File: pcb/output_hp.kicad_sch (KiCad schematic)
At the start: 1 part, among them J13 AudioJack3

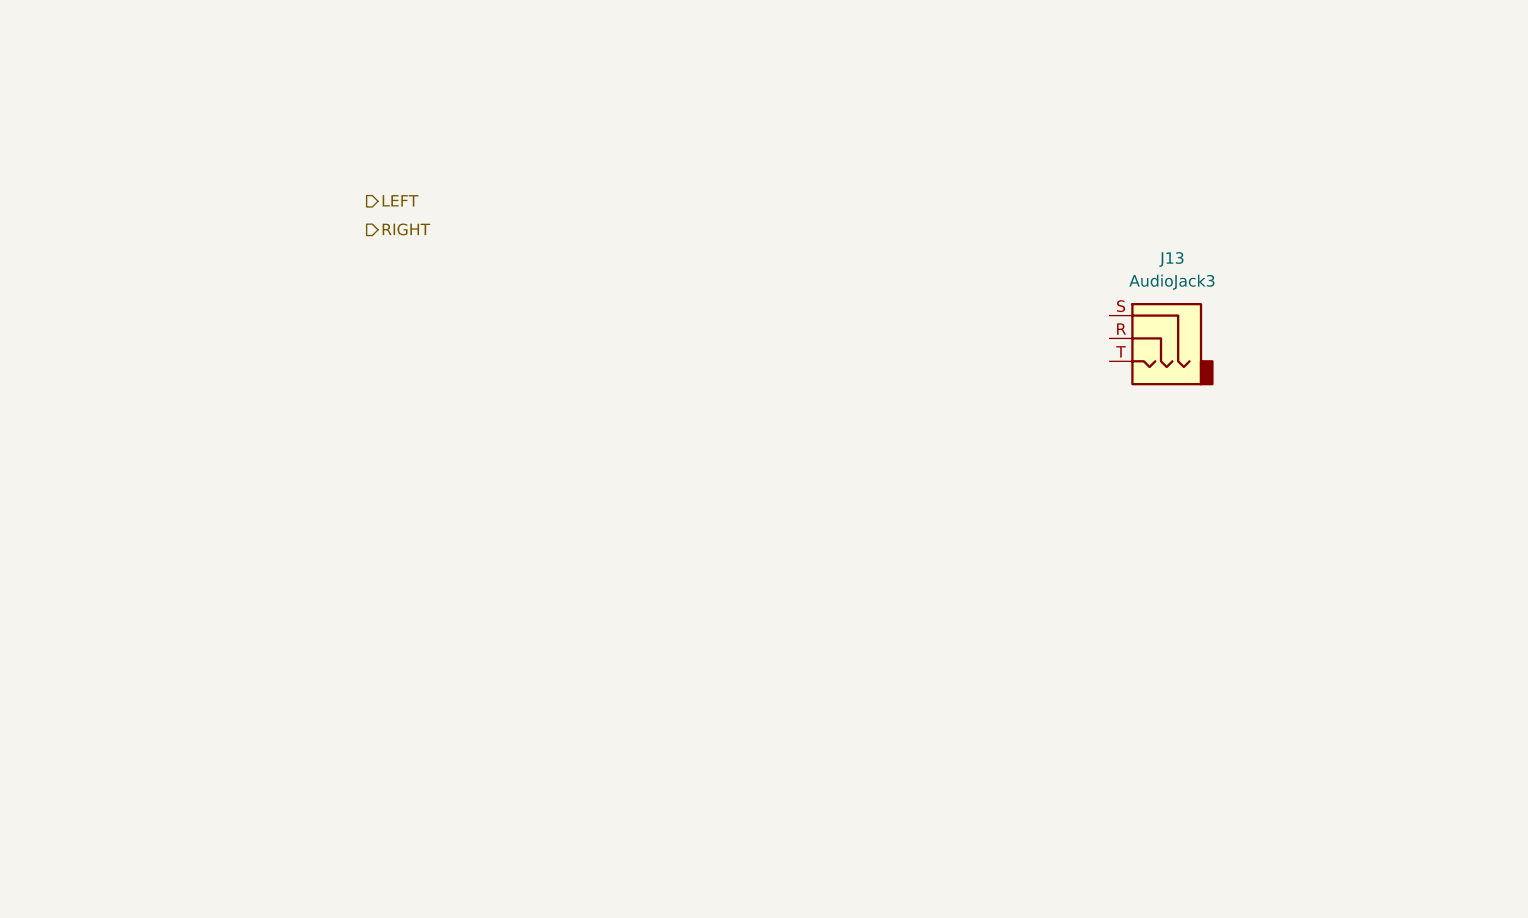
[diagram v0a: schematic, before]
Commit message: progress on hp
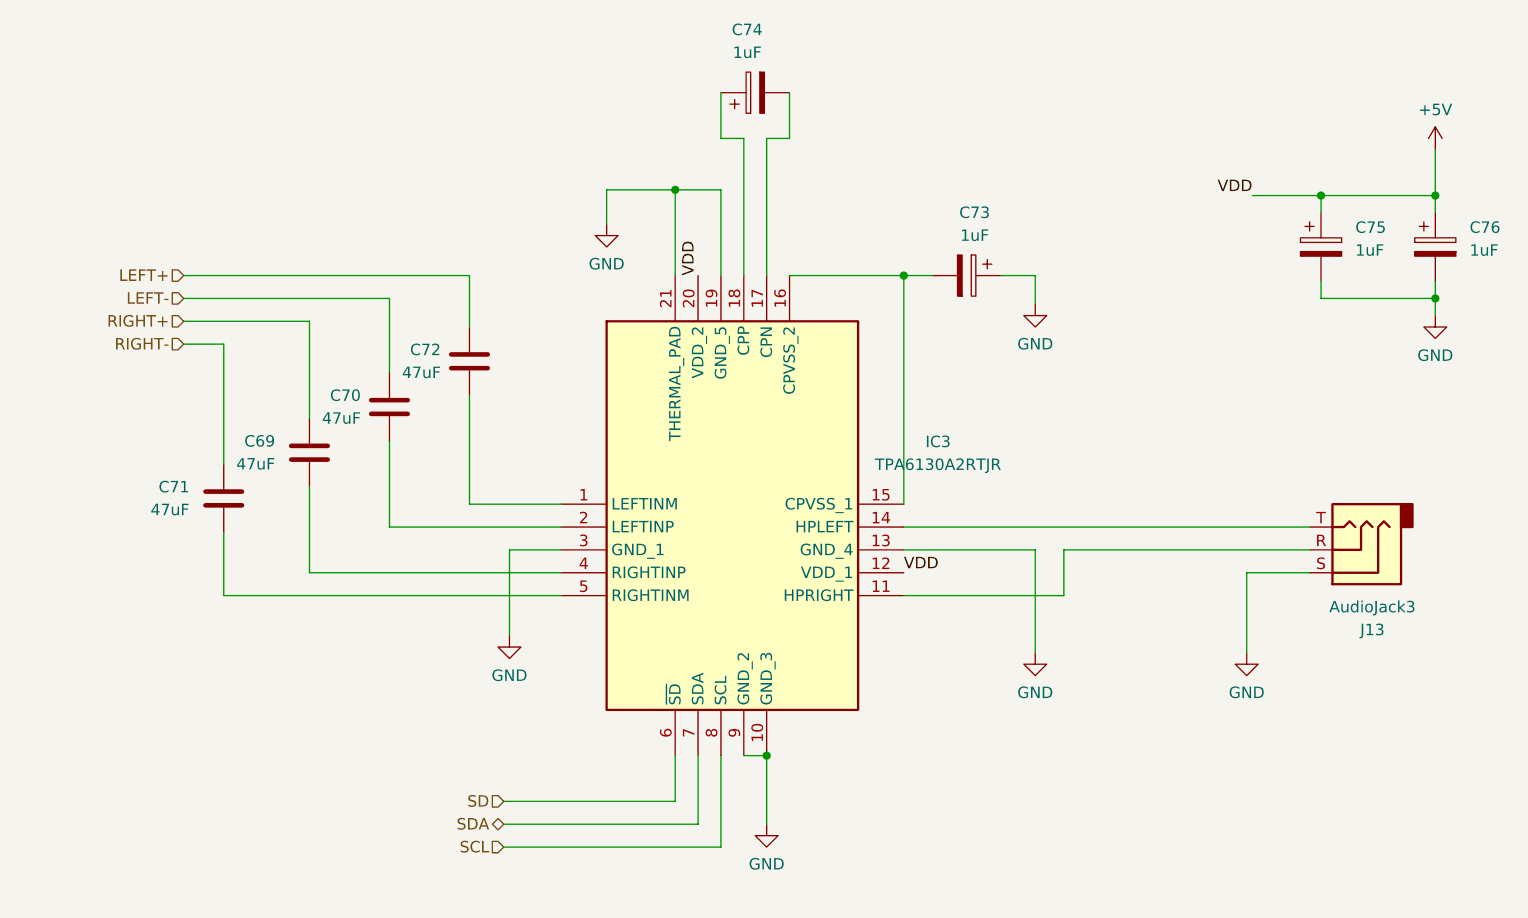
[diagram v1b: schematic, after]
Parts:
- added C69, C70, C71, C72: 47uF, symbol Device:C
- added C73, C74, C75, C76: 1uF, symbol Device:C_Polarized
- added IC3: TPA6130A2RTJR, QFN50P400X400X80-21N-D, symbol SamacSys_Parts:TPA6130A2RTJR
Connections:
- net at J13.R: now also IC3.11 (HPRIGHT)
- net GND: now reaches J13.S
- net GND: now also C73.1, C75.2, C76.2, IC3.10 (GND_3), IC3.13 (GND_4), IC3.19 (GND_5), IC3.21 (THERMAL_PAD), IC3.3 (GND_1), IC3.9 (GND_2)
- net at J13.T: now also IC3.14 (HPLEFT)
- new net: C72.1, IC3.1 (LEFTINM)
- new net: C73.2, IC3.15 (CPVSS_1), IC3.16 (CPVSS_2)
- new net: C74.2, IC3.17 (CPN)
- new net: C74.1, IC3.18 (CPP)
- new net: C70.1, IC3.2 (LEFTINP)
- new net: C69.2, IC3.4 (RIGHTINP)
- new net: C71.1, IC3.5 (RIGHTINM)
- new net +5V: C75.1, C76.1, IC3.12 (VDD_1), IC3.20 (VDD_2)
- new net LEFT+: C72.2
- new net LEFT-: C70.2
- new net RIGHT+: C69.1
- new net RIGHT-: C71.2
- new net SCL: IC3.8 (SCL)
- new net SD: IC3.6 (~{SD})
- new net SDA: IC3.7 (SDA)
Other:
- moved on the sheet: J13

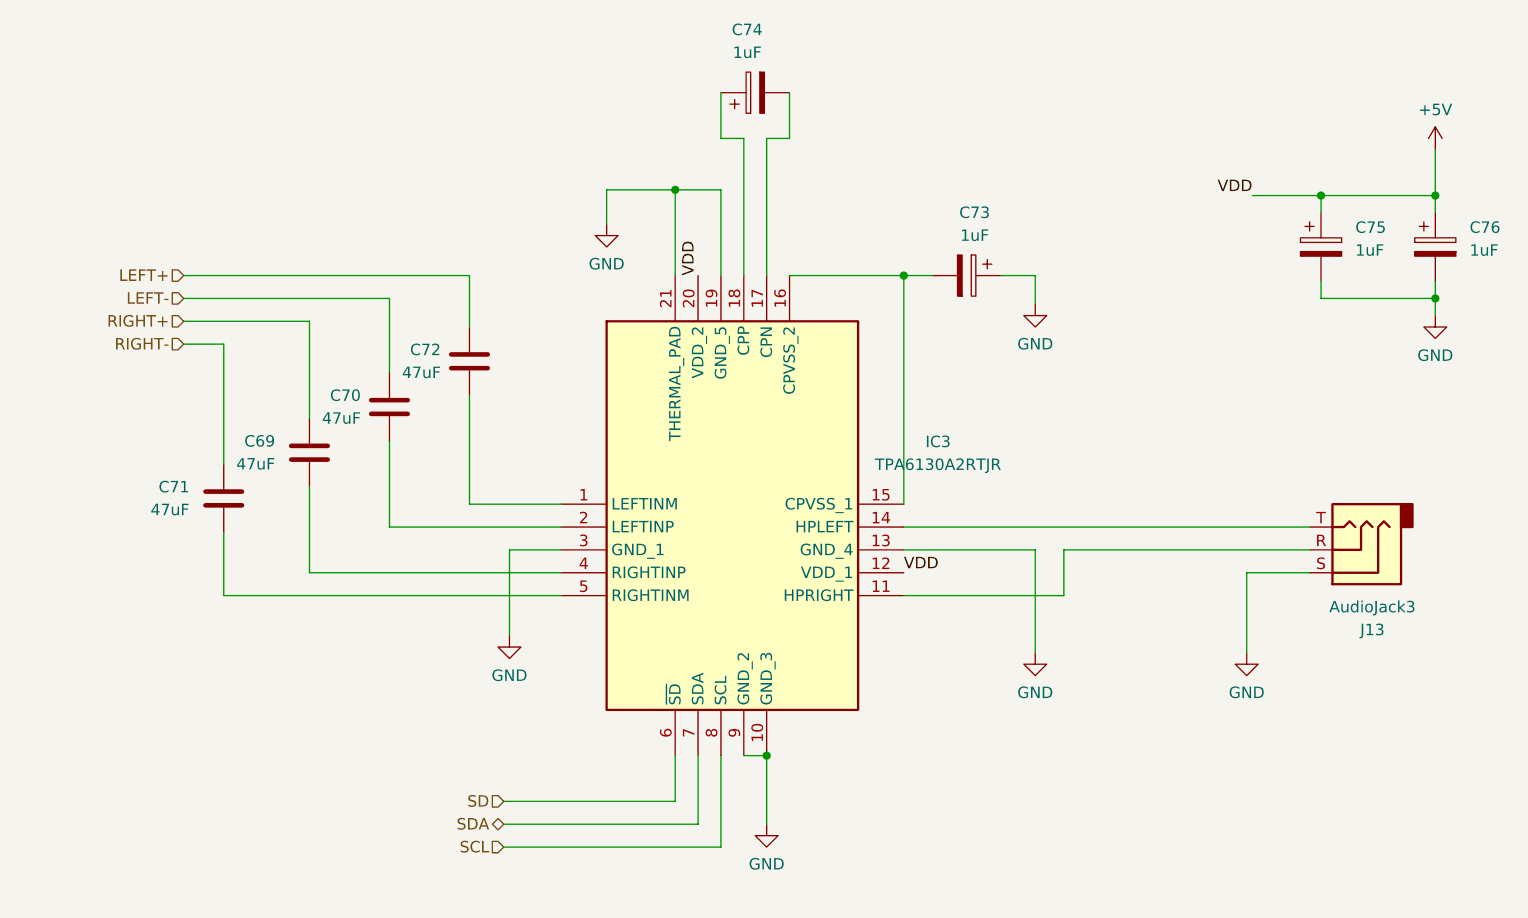
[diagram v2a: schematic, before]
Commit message: a lot of work! almost ready for rev
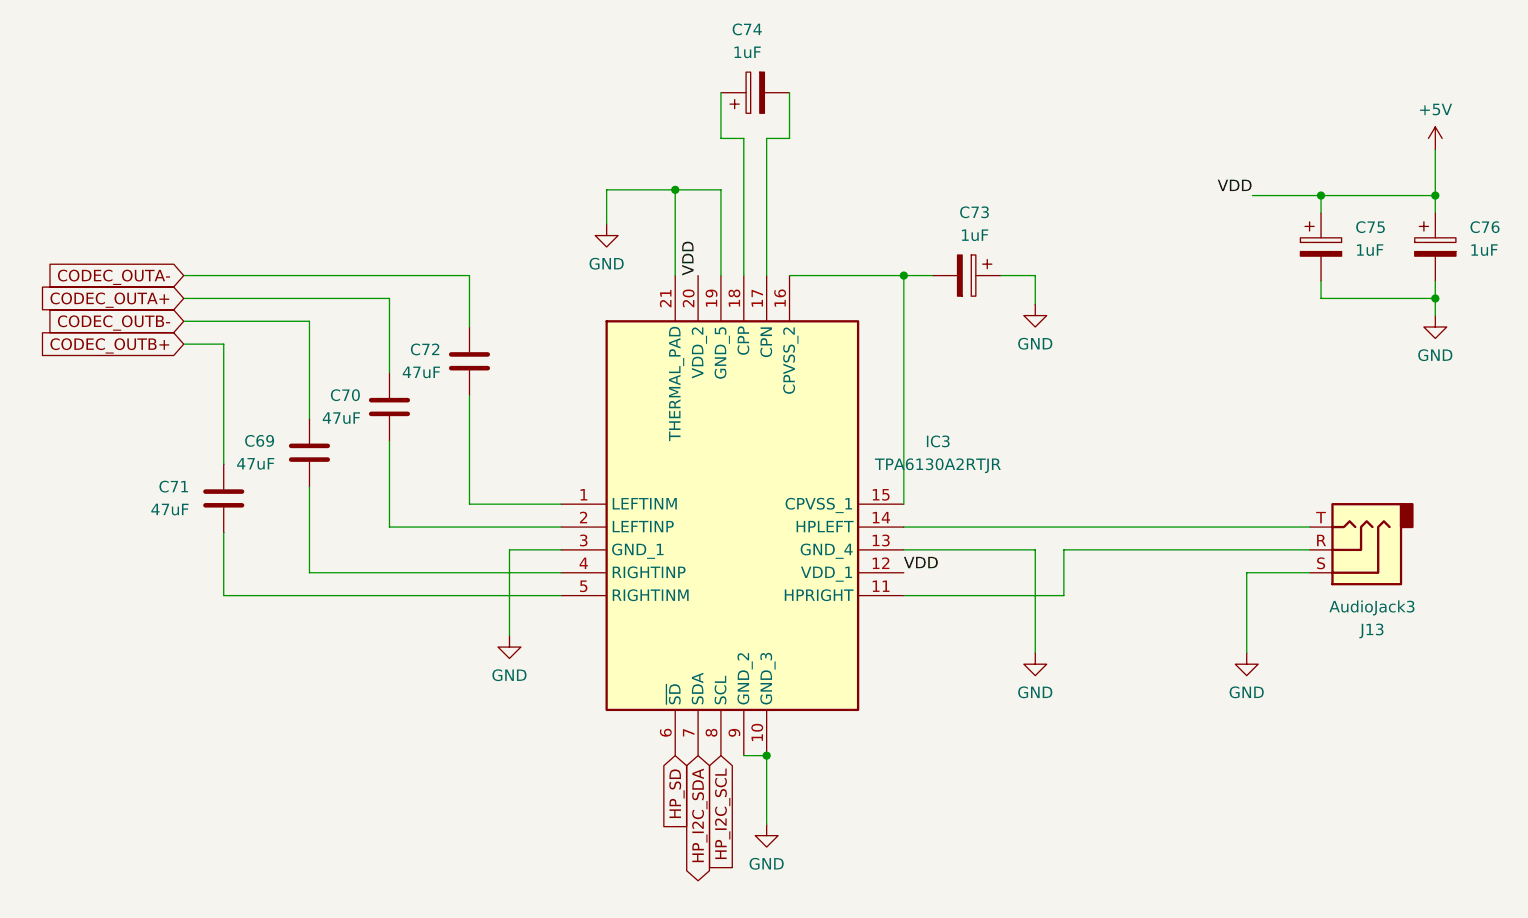
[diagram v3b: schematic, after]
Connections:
- net LEFT+ renamed CODEC_OUTA-
- net LEFT- renamed CODEC_OUTA+
- net RIGHT+ renamed CODEC_OUTB-
- net RIGHT- renamed CODEC_OUTB+
- net SCL renamed HP_I2C_SCL
- net SD renamed HP_SD
- net SDA renamed HP_I2C_SDA
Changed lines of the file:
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@@
-    (stroke (width 0) (type default))
-  )
-  (wire (pts (xy 130.81 118.745) (xy 130.81 126.365))
-    (stroke (width 0) (type default))
-  )
-  (wire (pts (xy 130.81 126.365) (xy 109.22 126.365))
     (stroke (width 0) (type default))
   )
@@
     (stroke (width 0) (type default))
   )
-  (wire (pts (xy 128.27 123.825) (xy 128.27 118.745))
-    (stroke (width 0) (type default))
-  )
   (wire (pts (xy 96.52 67.945) (xy 96.52 76.2))
     (stroke (width 0) (type default))
@@
     (stroke (width 0) (type default))
   )
-  (wire (pts (xy 109.22 128.905) (xy 133.35 128.905))
-    (stroke (width 0) (type default))
-  )
   (wire (pts (xy 153.67 93.345) (xy 198.755 93.345))
     (stroke (width 0) (type default))
@@
     (stroke (width 0) (type default))
   )
-  (wire (pts (xy 133.35 128.905) (xy 133.35 118.745))
-    (stroke (width 0) (type default))
-  )
   (wire (pts (xy 168.275 95.885) (xy 153.67 95.885))
     (stroke (width 0) (type default))
@@
   )
   (wire (pts (xy 87.63 70.485) (xy 87.63 81.28))
-    (stroke (width 0) (type default))
-  )
-  (wire (pts (xy 109.22 123.825) (xy 128.27 123.825))
     (stroke (width 0) (type default))
   )
@@
     (effects (font (size 1.27 1.27)) (justify left bottom))
   )
-  (hierarchical_label "SCL" (shape input) (at 109.22 128.905 180) (fields_autoplaced)
-    (effects (font (size 1.27 1.27)) (justify right))
-  )
-  (hierarchical_label "RIGHT-" (shape input) (at 73.66 73.025 180) (fields_autoplaced)
-    (effects (font (size 1.27 1.27)) (justify right))
-  )
-  (hierarchical_label "LEFT-" (shape input) (at 73.66 67.945 180) (fields_autoplaced)
-    (effects (font (size 1.27 1.27)) (justify right))
-  )
-  (hierarchical_label "LEFT+" (shape input) (at 73.66 65.405 180) (fields_autoplaced)
-    (effects (font (size 1.27 1.27)) (justify right))
-  )
-  (hierarchical_label "SD" (shape input) (at 109.22 123.825 180) (fields_autoplaced)
-    (effects (font (size 1.27 1.27)) (justify right))
-  )
-  (hierarchical_label "SDA" (shape bidirectional) (at 109.22 126.365 180) (fields_autoplaced)
-    (effects (font (size 1.27 1.27)) (justify right))
-  )
-  (hierarchical_label "RIGHT+" (shape input) (at 73.66 70.485 180) (fields_autoplaced)
-    (effects (font (size 1.27 1.27)) (justify right))
+  (global_label "CODEC_OUTA-" (shape input) (at 73.66 65.405 180) (fields_autoplaced)
+    (effects (font (size 1.27 1.27)) (justify right))
+    (property "Intersheetrefs" "${INTERSHEET_REFS}" (at 57.1281 65.405 0)
+      (effects (font (size 1.27 1.27)) (justify right) hide)
+    )
+  )
+  (global_label "HP_I2C_SDA" (shape bidirectional) (at 130.81 118.745 270) (fields_autoplaced)
+    (effects (font (size 1.27 1.27)) (justify right))
+    (property "Intersheetrefs" "${INTERSHEET_REFS}" (at 130.81 134.0296 90)
+      (effects (font (size 1.27 1.27)) (justify right) hide)
+    )
+  )
+  (global_label "CODEC_OUTA+" (shape input) (at 73.66 67.945 180) (fields_autoplaced)
+    (effects (font (size 1.27 1.27)) (justify right))
+    (property "Intersheetrefs" "${INTERSHEET_REFS}" (at 57.1281 67.945 0)
+      (effects (font (size 1.27 1.27)) (justify right) hide)
+    )
+  )
+  (global_label "CODEC_OUTB+" (shape input) (at 73.66 73.025 180) (fields_autoplaced)
+    (effects (font (size 1.27 1.27)) (justify right))
+    (property "Intersheetrefs" "${INTERSHEET_REFS}" (at 56.9467 73.025 0)
+      (effects (font (size 1.27 1.27)) (justify right) hide)
+    )
+  )
+  (global_label "HP_I2C_SCL" (shape input) (at 133.35 118.745 270) (fields_autoplaced)
+    (effects (font (size 1.27 1.27)) (justify right))
+    (property "Intersheetrefs" "${INTERSHEET_REFS}" (at 133.35 132.8578 90)
+      (effects (font (size 1.27 1.27)) (justify right) hide)
+    )
+  )
+  (global_label "CODEC_OUTB-" (shape input) (at 73.66 70.485 180) (fields_autoplaced)
+    (effects (font (size 1.27 1.27)) (justify right))
+    (property "Intersheetrefs" "${INTERSHEET_REFS}" (at 56.9467 70.485 0)
+      (effects (font (size 1.27 1.27)) (justify right) hide)
+    )
+  )
+  (global_label "HP_SD" (shape input) (at 128.27 118.745 270) (fields_autoplaced)
+    (effects (font (size 1.27 1.27)) (justify right))
+    (property "Intersheetrefs" "${INTERSHEET_REFS}" (at 128.27 127.7778 90)
+      (effects (font (size 1.27 1.27)) (justify right) hide)
+    )
   )
   (symbol (lib_id "Connector_Audio:AudioJack3") (at 203.835 95.885 180) (unit 1)
